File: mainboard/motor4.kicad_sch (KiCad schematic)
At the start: 12 parts, among them U4 DRV8323RSRGZT

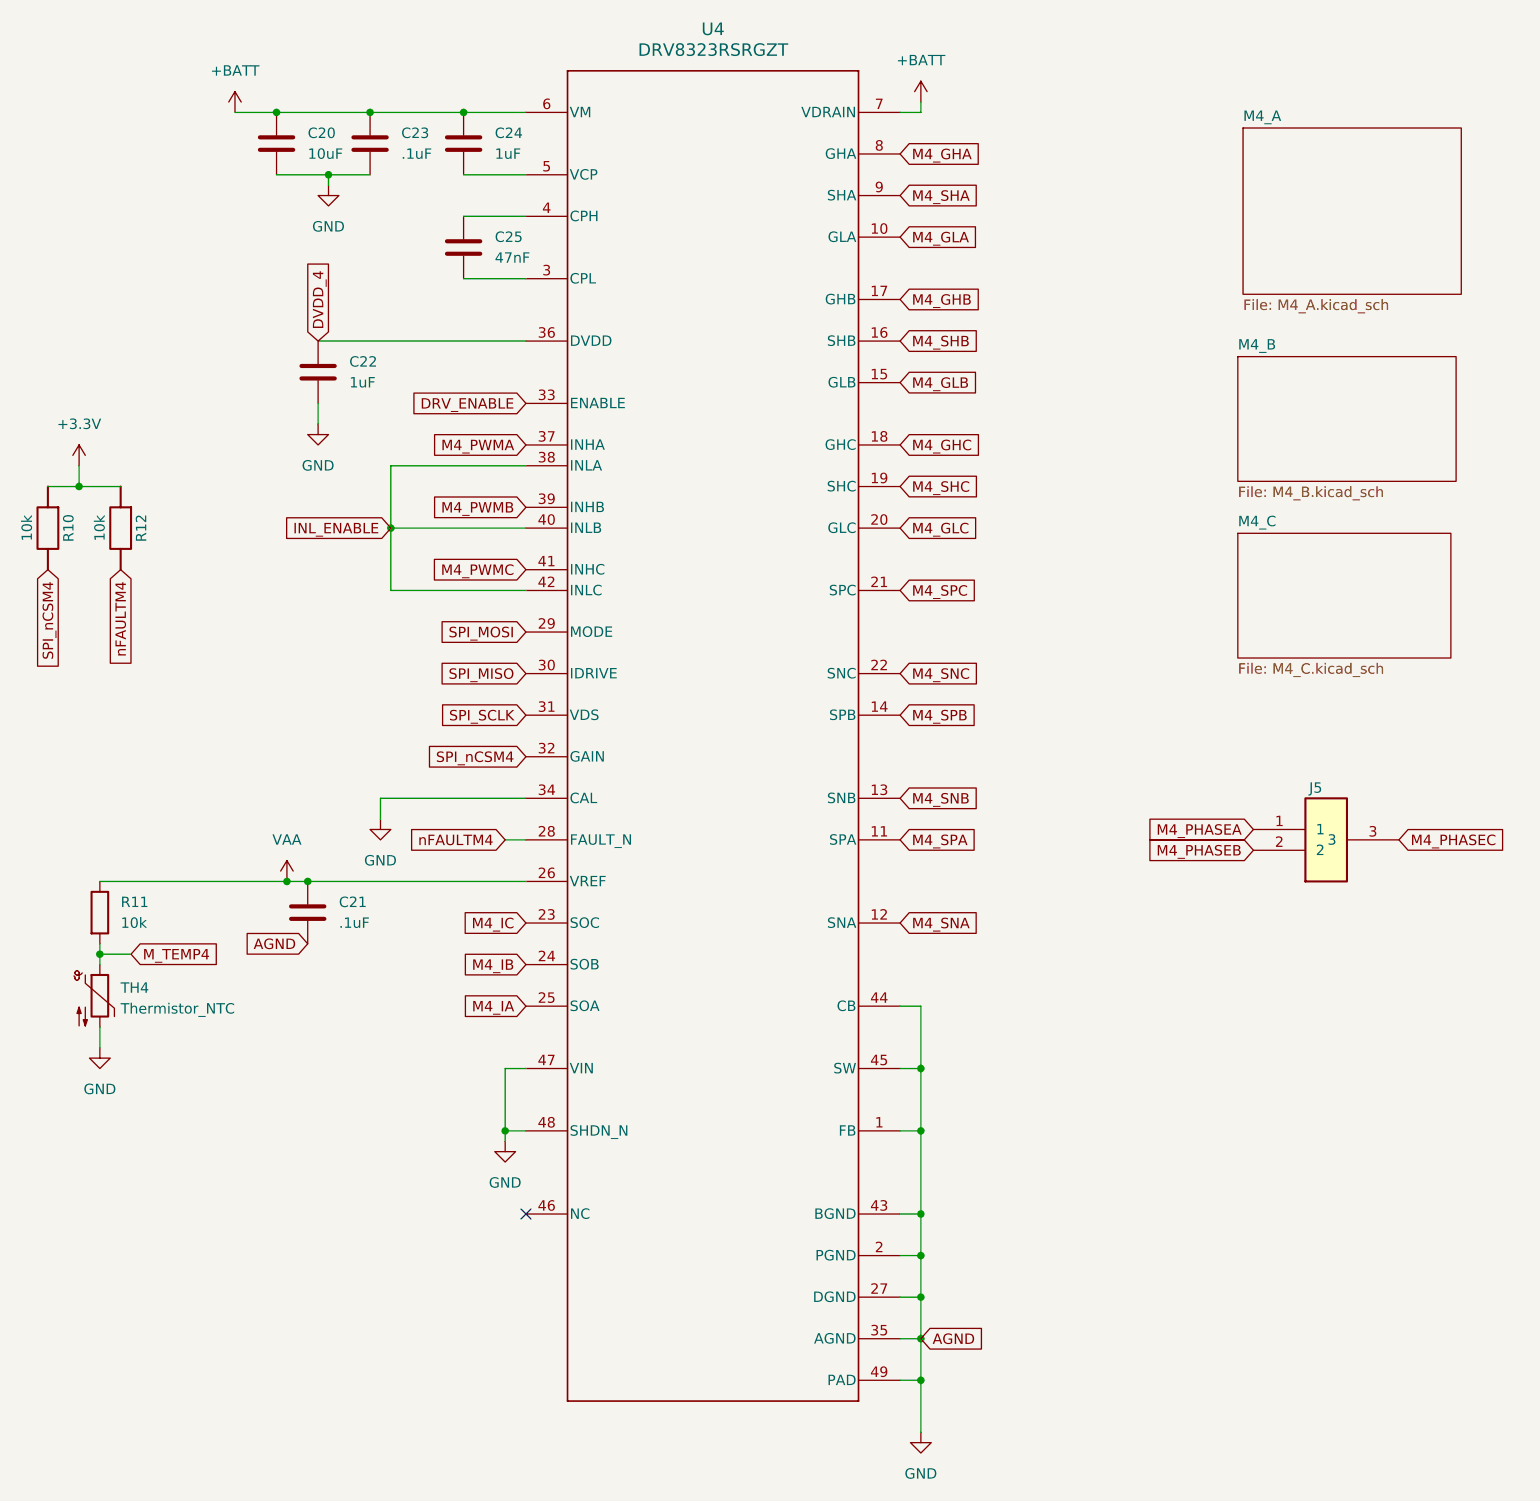
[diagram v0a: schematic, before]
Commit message: Initial layout completed
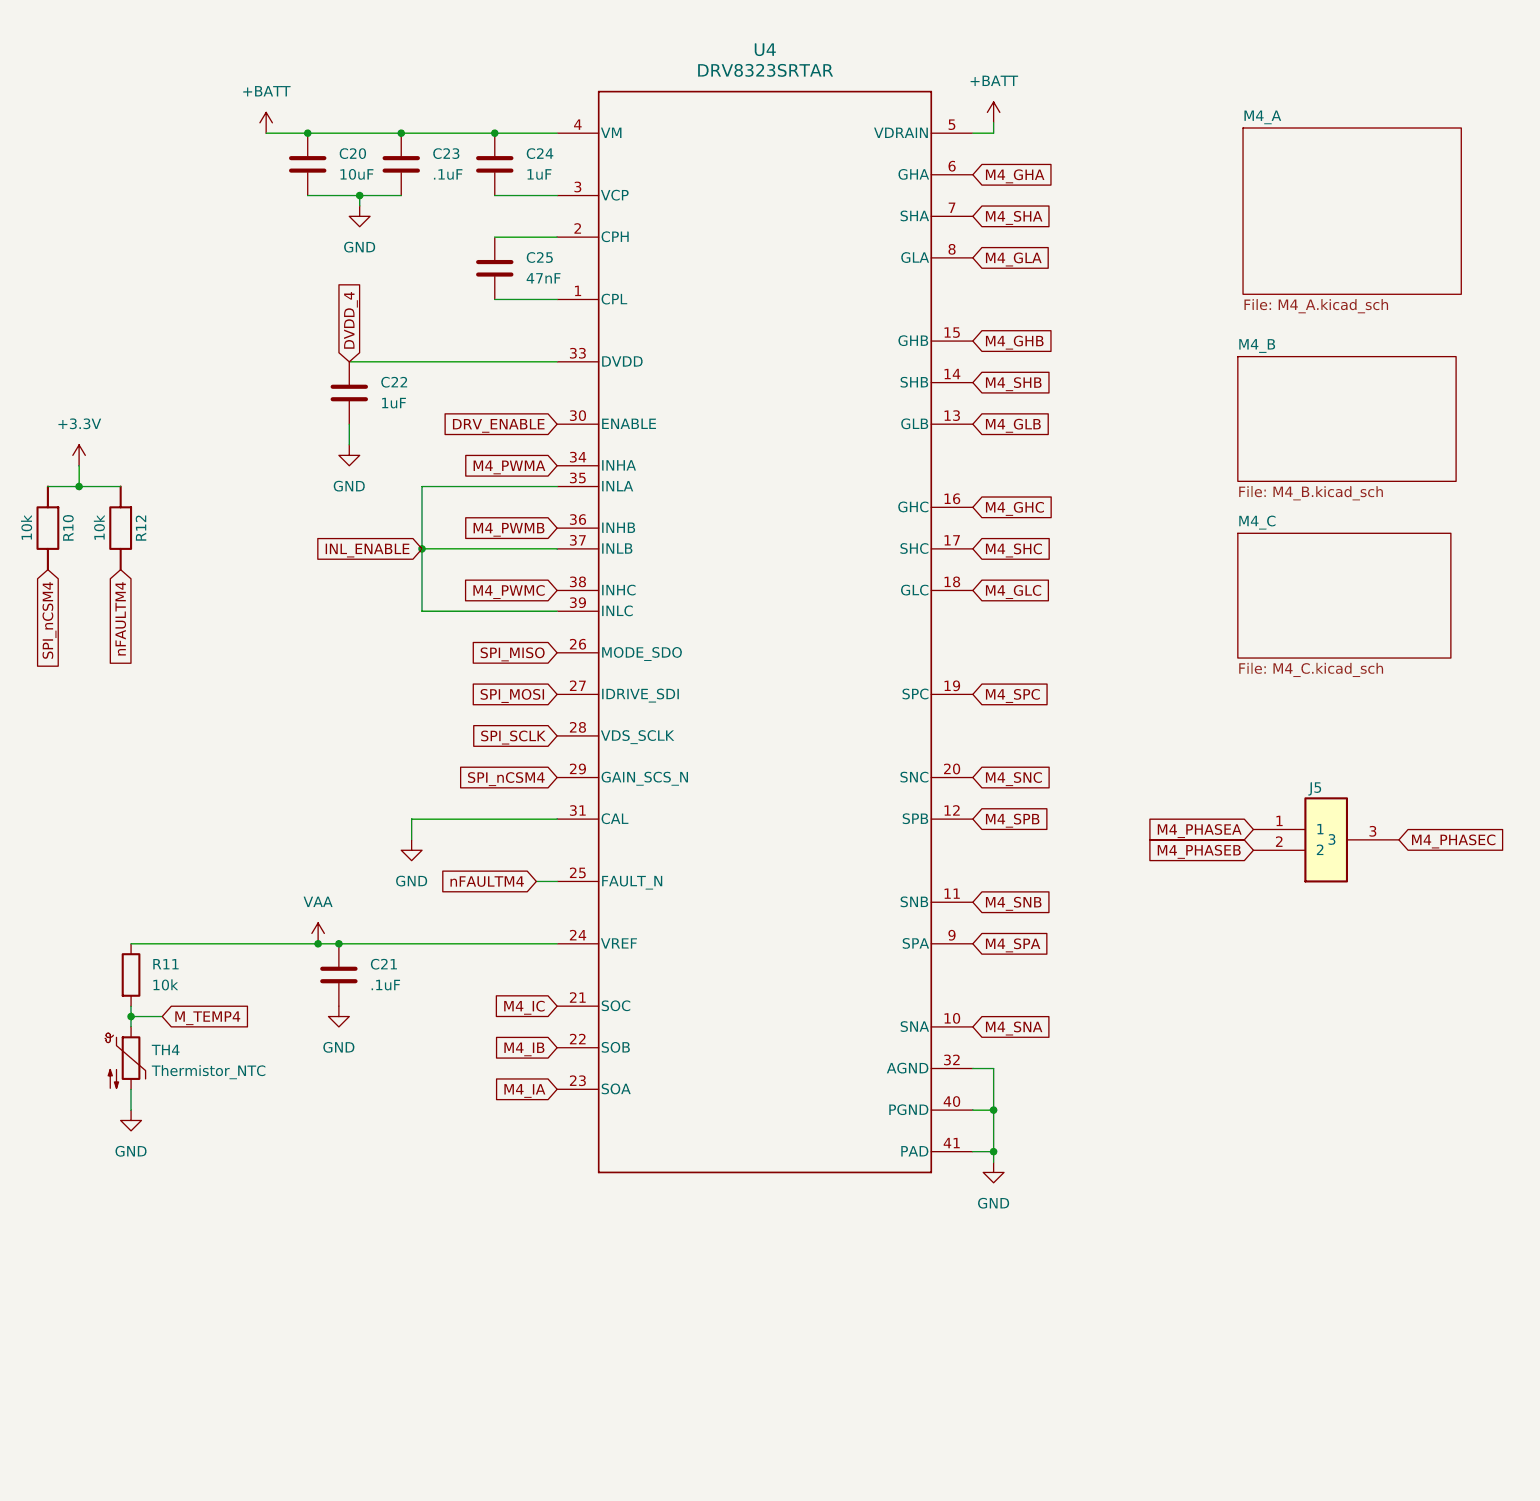
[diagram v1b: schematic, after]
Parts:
- removed U4: DRV8323RSRGZT, DRV8323RSRGZT_new:RGZ0048A, symbol DRV8323RSRGZT_new:DRV8323RSRGZT
- added U4: DRV8323SRTAR, DRV8323SRTAR:RTA0040B_NV, symbol DRV8323SR:DRV8323SRTAR
- C20: footprint Capacitor_SMD:C_1210_3225Metric -> Capacitor_SMD:C_1206_3216Metric
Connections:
- net +BATT: now also U4.4 (VM), U4.5 (VDRAIN)
- net DRV_ENABLE: now also U4.30 (ENABLE)
- net DVDD_4: now also U4.33 (DVDD)
- net GND: now also U4.31 (CAL), U4.32 (AGND), U4.40 (PGND), U4.41 (PAD)
- net INL_ENABLE: now also U4.35 (INLA), U4.37 (INLB), U4.39 (INLC)
- net M4_GHA: now also U4.6 (GHA)
- net M4_GHB: now also U4.15 (GHB)
- net M4_GHC: now also U4.16 (GHC)
- net M4_GLA: now also U4.8 (GLA)
- net M4_GLB: now also U4.13 (GLB)
- net M4_GLC: now also U4.18 (GLC)
- net M4_IA: now also U4.23 (SOA)
- net M4_IB: now also U4.22 (SOB)
- net M4_IC: now also U4.21 (SOC)
- net M4_PWMA: now also U4.34 (INHA)
- net M4_PWMB: now also U4.36 (INHB)
- net M4_PWMC: now also U4.38 (INHC)
- net M4_SHA: now also U4.7 (SHA)
- net M4_SHB: now also U4.14 (SHB)
- net M4_SHC: now also U4.17 (SHC)
- net M4_SNA: now also U4.10 (SNA)
- net M4_SNB: now also U4.11 (SNB)
- net M4_SNC: now also U4.20 (SNC)
- net M4_SPA: now also U4.9 (SPA)
- net M4_SPB: now also U4.12 (SPB)
- net M4_SPC: now also U4.19 (SPC)
- net SPI_MISO: now also U4.26 (MODE_SDO)
- net SPI_MOSI: now also U4.27 (IDRIVE_SDI)
- net SPI_SCLK: now also U4.28 (VDS_SCLK)
- net SPI_nCSM4: now also U4.29 (GAIN_SCS_N)
- net VAA: now also U4.24 (VREF)
- net nFAULTM4: now also U4.25 (FAULT_N)
- net at C25.1: now also U4.2 (CPH)
- net at C25.2: now also U4.1 (CPL)
- net at C24.2: now also U4.3 (VCP)
- no-connect marks 1 -> 0
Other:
- moved on the sheet: C20, C21, C22, C23, C24, C25, R11, TH4
